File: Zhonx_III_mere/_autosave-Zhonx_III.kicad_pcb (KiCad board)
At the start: 2 copper layers, 133 parts, among them K1 L_Motor, K2 R_Motor, K3 USART, P1 JTAG, Q1 FDV301N, Q2 FDV301N, U1 MCP73213, U10 BSL214N, U11 BSL214N, U12 24LC64T, U14 STM32F405RGT6, U16 Line_1, U17 Line_2, U18 Line_3, U19 Line_4, U2 A3918, U20 Line_5, U3 A3918, U4 LTC2955CTS8-2, U5 SIB911DK, U6 SI1551DL, U7 LM2940, U8 MCP1700, U9 MCP1700, X1 16MHz

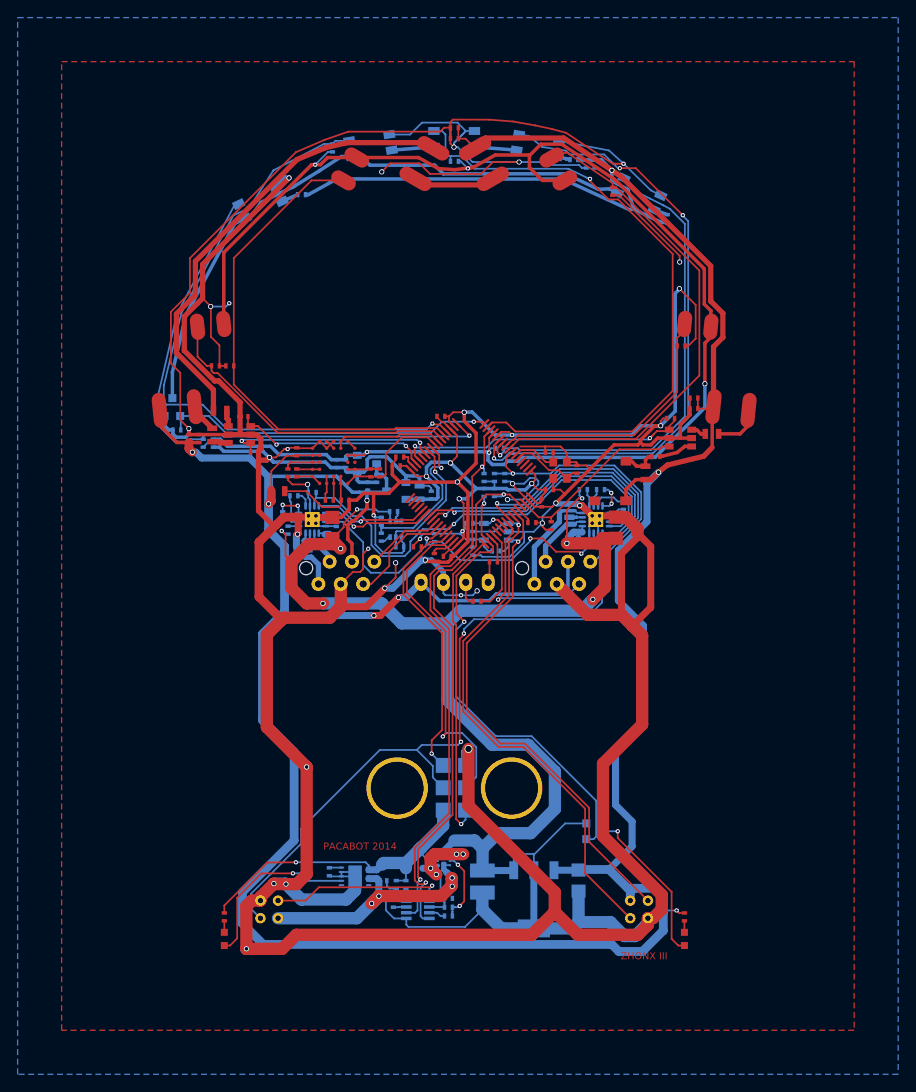
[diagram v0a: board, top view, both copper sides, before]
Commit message: Nouvelle librairie (.pretty)
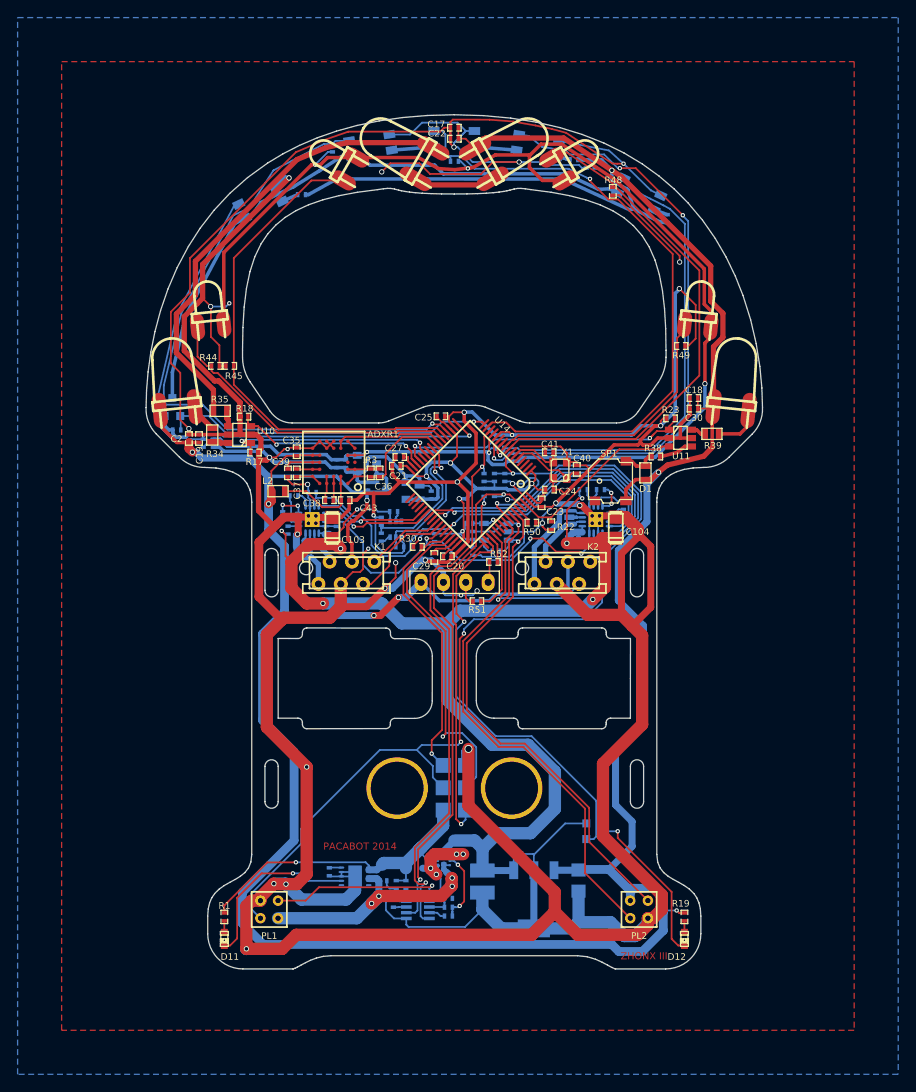
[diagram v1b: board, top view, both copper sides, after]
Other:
- board outline added: 70 x 97 mm
